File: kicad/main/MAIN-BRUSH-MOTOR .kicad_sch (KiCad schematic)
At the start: 7 parts, among them U20 DRV8870DDAR

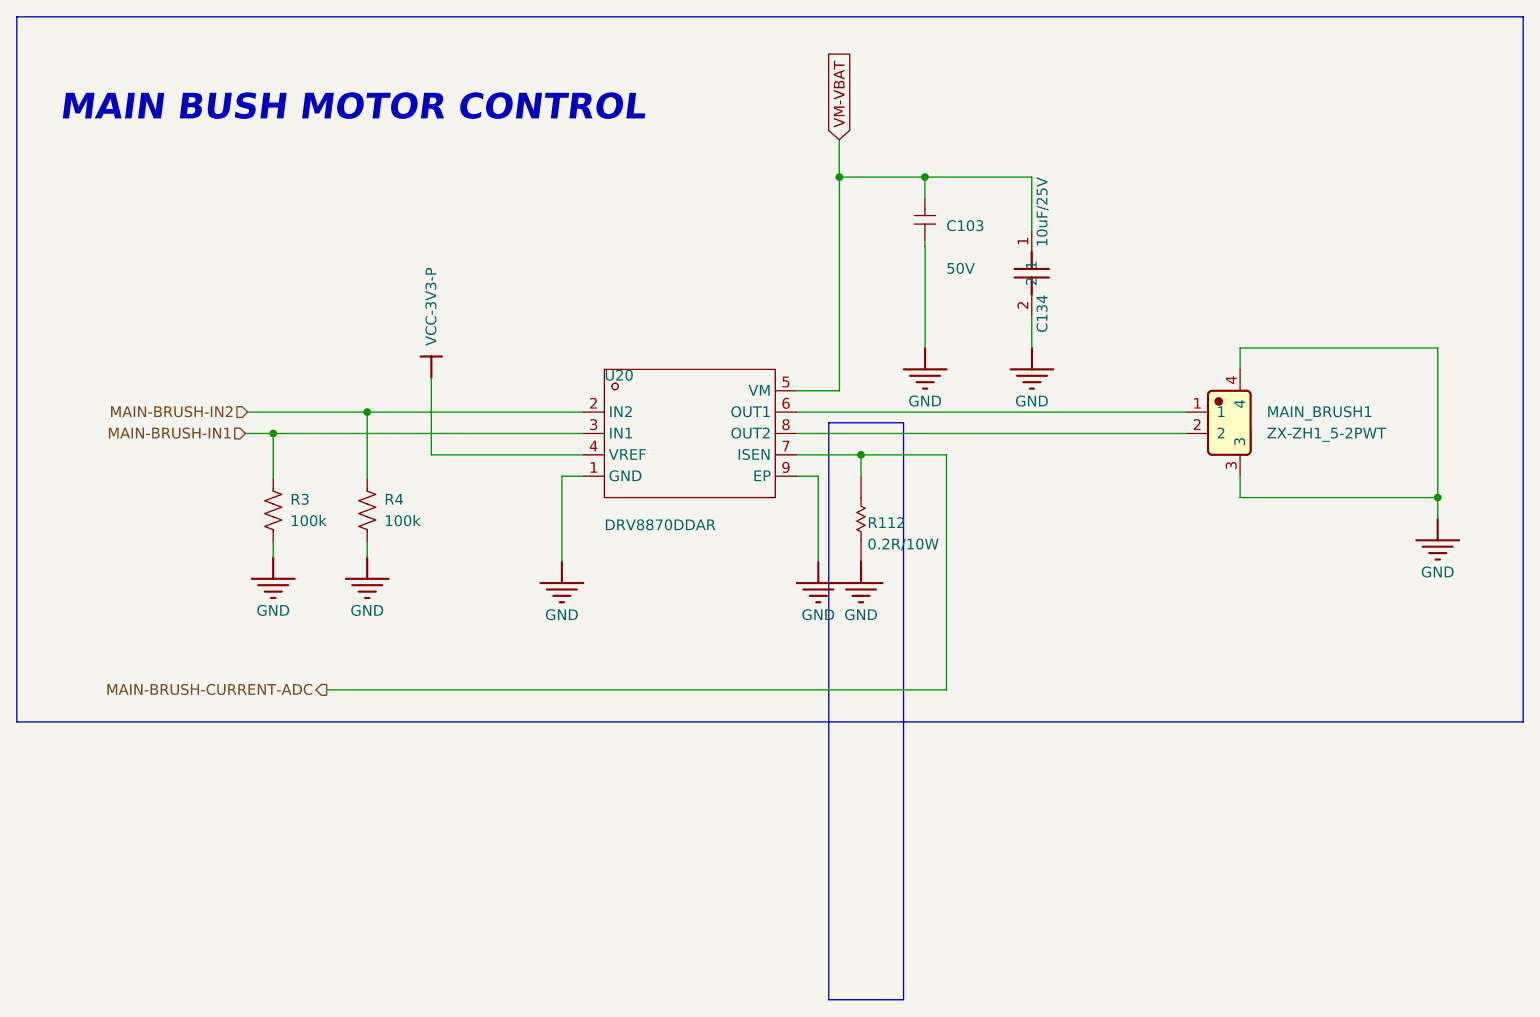
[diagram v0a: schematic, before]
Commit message: Second review round
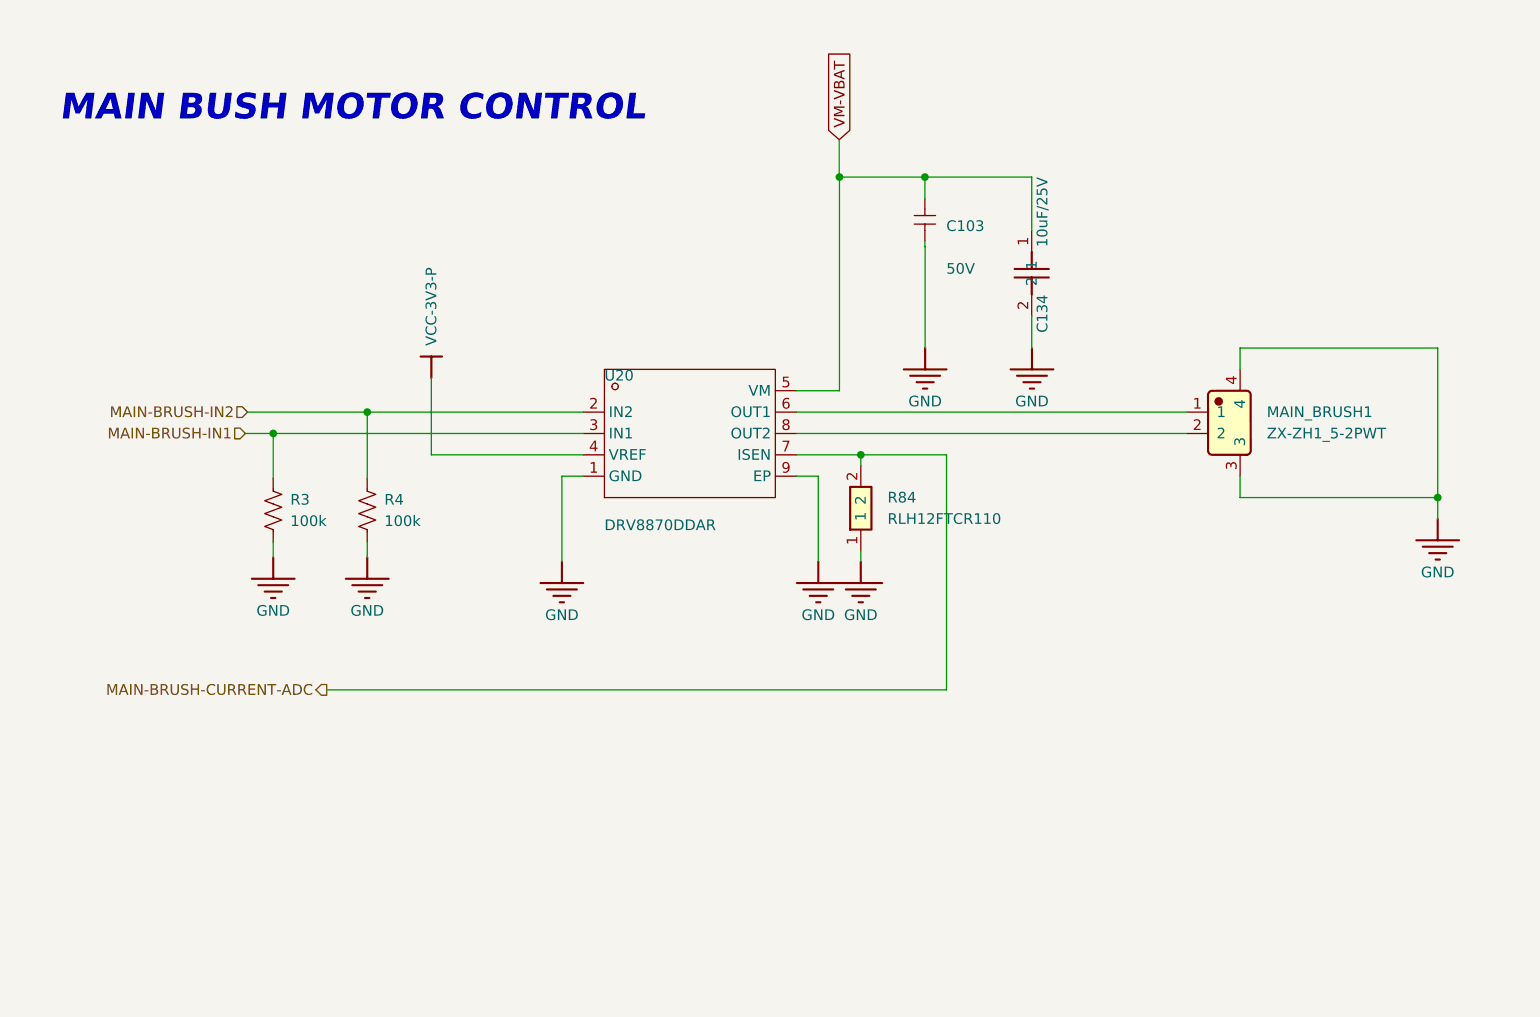
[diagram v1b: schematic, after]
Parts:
- removed R112: 0.2R/10W, Resistor_SMD:R_2512_6332Metric, symbol DesignLibrary:WHEEL MOTOR_1_Resistor-1_DesignLibrary.SchLib
- added R84: RLH12FTCR110, JLCImport:RLH12FTCR110, symbol JLCImport:RLH12FTCR110
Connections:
- net GND: now also R84.1
- net MAIN-BRUSH-CURRENT-ADC: now also R84.2
